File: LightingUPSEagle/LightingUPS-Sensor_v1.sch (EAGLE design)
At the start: 1 part

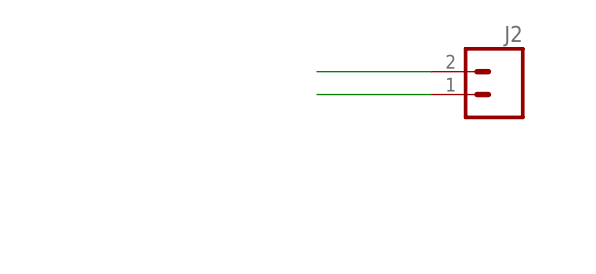
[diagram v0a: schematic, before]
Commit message: Add files via upload
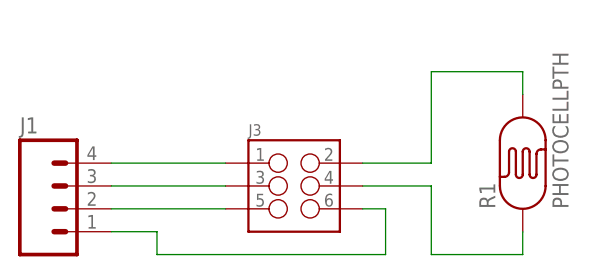
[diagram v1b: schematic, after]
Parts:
- removed J2: (no value), SparkFun-Connectors:M02PTH
- added J1: (no value), SparkFun-Connectors:M04PTH
- added J3: (no value), SparkFun-Connectors:M03X2SHROUD
- added R1: PHOTOCELLPTH, SparkFun-Sensors:PHOTOCELLPTH
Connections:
- new net N$5: J1.4, J3.1
- new net N$6: J1.3, J3.3
- new net N$7: J1.2, J3.5
- new net N$8: J1.1, J3.6
- net N$1: now also J3.4, R1.P$1; no longer J2.2
- net N$2: now also J3.2, R1.P$2; no longer J2.1
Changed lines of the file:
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@@
 </classes>
 <parts>
-<part name="J2" library="SparkFun-Connectors" deviceset="M02" device="PTH"/>
+<part name="R1" library="SparkFun-Sensors" deviceset="PHOTOCELL" device="PTH"/>
+<part name="J1" library="SparkFun-Connectors" deviceset="M04" device="PTH"/>
+<part name="J3" library="SparkFun-Connectors" deviceset="M03X2" device="SHROUD"/>
 </parts>
 <sheets>
@@
 </plain>
 <instances>
-<instance part="J2" gate="G$1" x="48.26" y="96.52" rot="MR0"/>
+<instance part="R1" gate="G$1" x="50.8" y="88.9" rot="R90"/>
+<instance part="J1" gate="G$1" x="0" y="83.82"/>
+<instance part="J3" gate="G$1" x="25.4" y="86.36"/>
 </instances>
 <busses>
@@
 <net name="N$1" class="0">
 <segment>
-<pinref part="J2" gate="G$1" pin="2"/>
-<wire x1="27.94" y1="99.06" x2="40.64" y2="99.06" width="0.1524" layer="91"/>
+<pinref part="J3" gate="G$1" pin="4"/>
+<wire x1="33.02" y1="86.36" x2="40.64" y2="86.36" width="0.1524" layer="91"/>
+<wire x1="40.64" y1="86.36" x2="40.64" y2="78.74" width="0.1524" layer="91"/>
+<pinref part="R1" gate="G$1" pin="P$1"/>
+<wire x1="40.64" y1="78.74" x2="50.8" y2="78.74" width="0.1524" layer="91"/>
+<wire x1="50.8" y1="78.74" x2="50.8" y2="81.28" width="0.1524" layer="91"/>
 </segment>
 </net>
 <net name="N$2" class="0">
 <segment>
-<pinref part="J2" gate="G$1" pin="1"/>
-<wire x1="27.94" y1="96.52" x2="40.64" y2="96.52" width="0.1524" layer="91"/>
+<pinref part="J3" gate="G$1" pin="2"/>
+<wire x1="33.02" y1="88.9" x2="40.64" y2="88.9" width="0.1524" layer="91"/>
+<wire x1="40.64" y1="88.9" x2="40.64" y2="99.06" width="0.1524" layer="91"/>
+<pinref part="R1" gate="G$1" pin="P$2"/>
+<wire x1="40.64" y1="99.06" x2="50.8" y2="99.06" width="0.1524" layer="91"/>
+<wire x1="50.8" y1="99.06" x2="50.8" y2="96.52" width="0.1524" layer="91"/>
 </segment>
 </net>
+<net name="N$5" class="0">
+<segment>
+<pinref part="J1" gate="G$1" pin="4"/>
+<pinref part="J3" gate="G$1" pin="1"/>
+<wire x1="5.08" y1="88.9" x2="17.78" y2="88.9" width="0.1524" layer="91"/>
+</segment>
+</net>
+<net name="N$6" class="0">
+<segment>
+<pinref part="J1" gate="G$1" pin="3"/>
+<pinref part="J3" gate="G$1" pin="3"/>
+<wire x1="5.08" y1="86.36" x2="17.78" y2="86.36" width="0.1524" layer="91"/>
+</segment>
+</net>
+<net name="N$7" class="0">
+<segment>
+<pinref part="J1" gate="G$1" pin="2"/>
+<pinref part="J3" gate="G$1" pin="5"/>
+<wire x1="5.08" y1="83.82" x2="17.78" y2="83.82" width="0.1524" layer="91"/>
+</segment>
+</net>
+<net name="N$8" class="0">
+<segment>
+<pinref part="J1" gate="G$1" pin="1"/>
+<wire x1="5.08" y1="81.28" x2="10.16" y2="81.28" width="0.1524" layer="91"/>
+<wire x1="10.16" y1="81.28" x2="10.16" y2="78.74" width="0.1524" layer="91"/>
+<wire x1="10.16" y1="78.74" x2="35.56" y2="78.74" width="0.1524" layer="91"/>
+<wire x1="35.56" y1="78.74" x2="35.56" y2="83.82" width="0.1524" layer="91"/>
+<pinref part="J3" gate="G$1" pin="6"/>
+<wire x1="35.56" y1="83.82" x2="33.02" y2="83.82" width="0.1524" layer="91"/>
+</segment>
+</net>
